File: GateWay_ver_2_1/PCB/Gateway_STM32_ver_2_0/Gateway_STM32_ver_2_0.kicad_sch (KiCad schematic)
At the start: 44 parts, among them J4 Conn_01x04, SW2 SW_Push, U7 STM32F407VETx, Y1 8mhz, Y2 Crystal_GND23

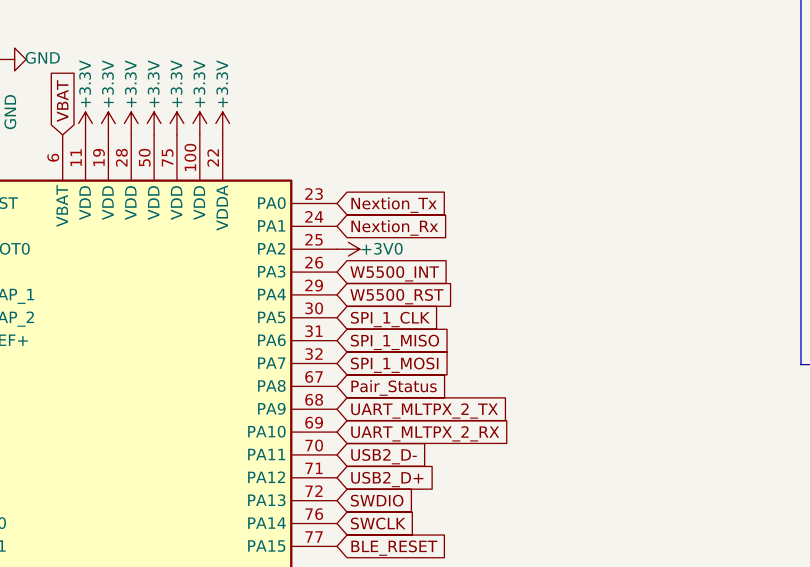
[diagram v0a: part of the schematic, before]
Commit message: 1
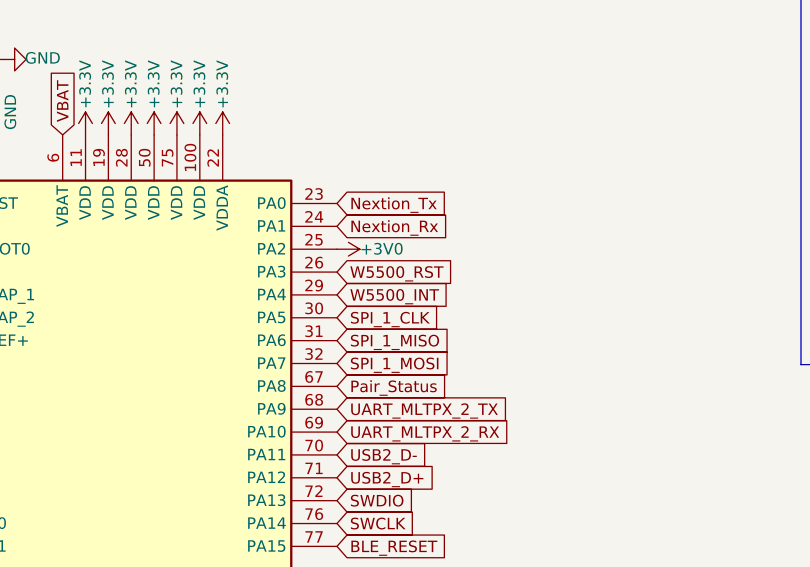
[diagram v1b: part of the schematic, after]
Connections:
- net W5500_INT: now also U7.29 (PA4); no longer U7.26 (PA3)
- net W5500_RST: now also U7.26 (PA3); no longer U7.29 (PA4)
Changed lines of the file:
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@@
     )
   )
-  (global_label "W5500_RST" (shape input) (at 114.046 61.468 0) (fields_autoplaced)
+  (global_label "W5500_RST" (shape input) (at 114.046 58.928 0) (fields_autoplaced)
     (effects (font (size 1.27 1.27)) (justify left))
-    (property "Intersheet References" "${INTERSHEET_REFS}" (id 0) (at 127.0745 61.5474 0)
+    (property "Intersheet References" "${INTERSHEET_REFS}" (id 0) (at 127.0745 59.0074 0)
       (effects (font (size 1.27 1.27)) (justify left) hide)
     )
@@
     )
   )
-  (global_label "W5500_INT" (shape input) (at 114.046 58.928 0) (fields_autoplaced)
+  (global_label "W5500_INT" (shape input) (at 114.046 61.468 0) (fields_autoplaced)
     (effects (font (size 1.27 1.27)) (justify left))
-    (property "Intersheet References" "${INTERSHEET_REFS}" (id 0) (at 126.5302 59.0074 0)
+    (property "Intersheet References" "${INTERSHEET_REFS}" (id 0) (at 126.5302 61.5474 0)
       (effects (font (size 1.27 1.27)) (justify left) hide)
     )
@@
       (reference "#PWR0291") (unit 1) (value "+3V0") (footprint "")
     )
+    (path "/8600ef7b-7ca3-4a98-82a9-dc0d4d9efebb/718c0a71-8caf-4775-a9fd-8fc71bd22381"
+      (reference "#PWR0292") (unit 1) (value "GND") (footprint "")
+    )
     (path "/17dbbc3f-e526-4f0c-aeef-1a51fbd344a5/44e527b0-0c19-4642-86b3-bad529530e43"
       (reference "#PWR0319") (unit 1) (value "+5V") (footprint "")
@@
       (reference "C27") (unit 1) (value "100uF") (footprint "Capacitor_SMD:C_1210_3225Metric")
     )
+    (path "/8600ef7b-7ca3-4a98-82a9-dc0d4d9efebb/57ebf0ae-ce32-4e87-bcc0-a3c92ff85e2b"
+      (reference "C28") (unit 1) (value "0.1uF") (footprint "Capacitor_SMD:C_0603_1608Metric")
+    )
     (path "/ddd7290c-9338-4156-8fc4-c8c1045ba903/431b55cc-a9c8-4999-8c91-373433ab34f0"
       (reference "C29") (unit 1) (value "0.1uF") (footprint "Capacitor_SMD:C_0603_1608Metric")
@@
       (reference "R93") (unit 1) (value "10k") (footprint "Resistor_SMD:R_0603_1608Metric")
     )
+    (path "/a04ecede-d1be-4f19-bba9-9cd40a161111/3f9a155b-ff8a-4cf2-8a3d-a6361ab24ec5"
+      (reference "R94") (unit 1) (value "0R") (footprint "Resistor_SMD:R_0603_1608Metric")
+    )
+    (path "/a04ecede-d1be-4f19-bba9-9cd40a161111/d410bbe8-62ea-4bf7-8bbe-58ba1610af3b"
+      (reference "R95") (unit 1) (value "0R") (footprint "Resistor_SMD:R_0603_1608Metric")
+    )
     (path "/dd619e6a-a0e1-4beb-8356-bcf75161c392/577f4706-5d40-4538-9616-d5b6ad5ea9f6"

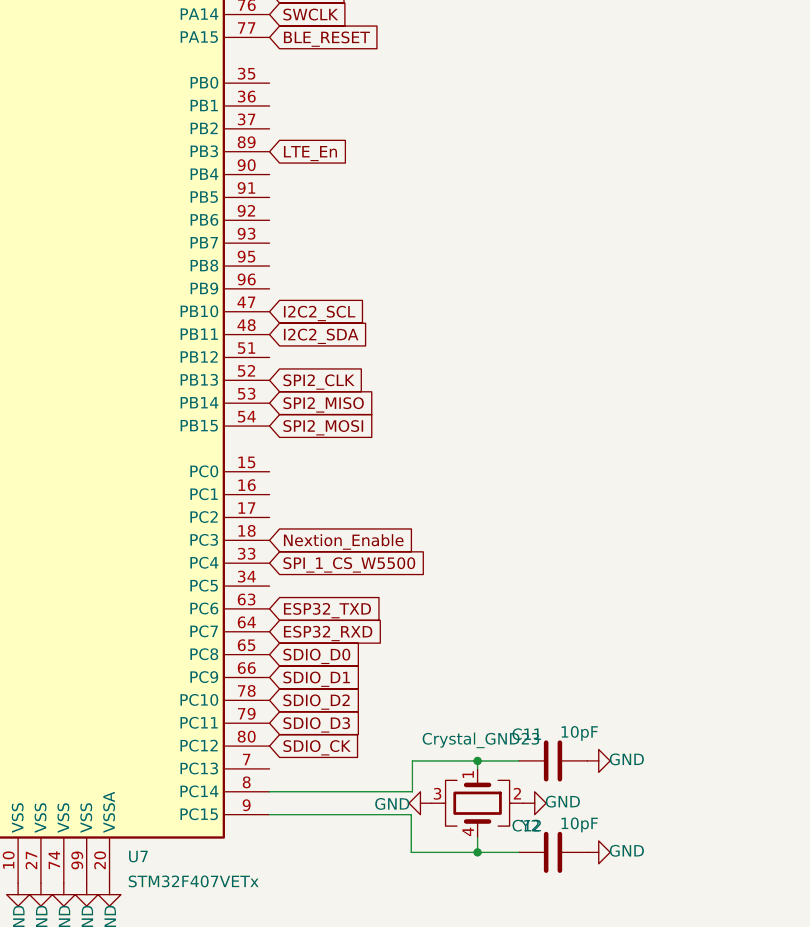
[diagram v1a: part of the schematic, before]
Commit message: 1
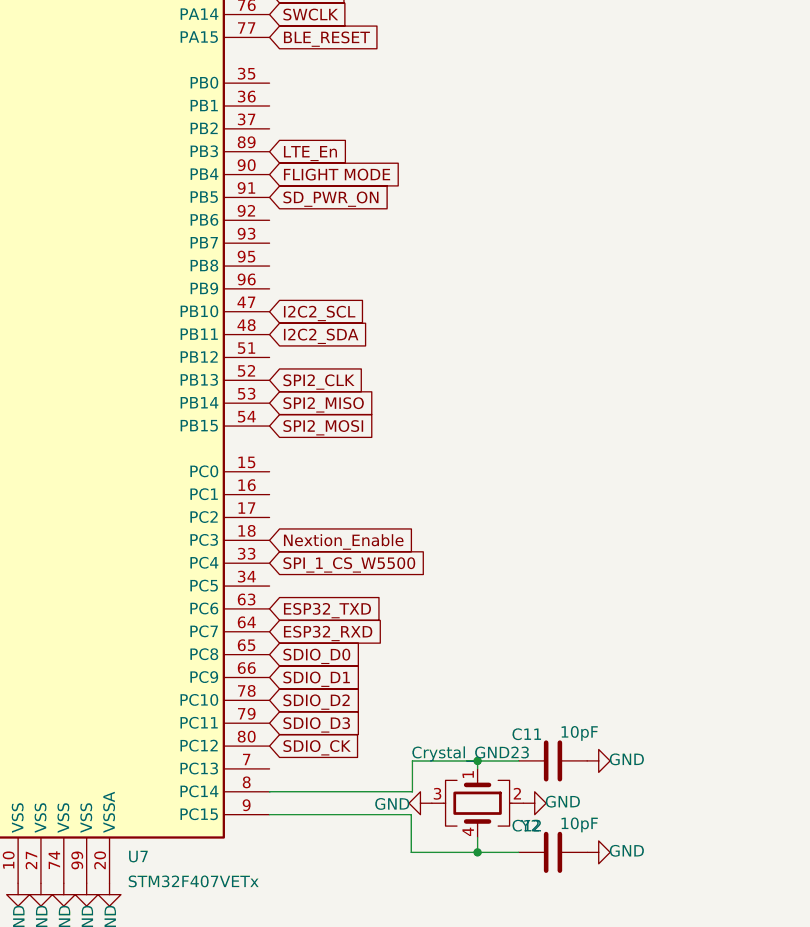
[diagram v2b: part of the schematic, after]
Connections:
- net FLIGHT MODE: now reaches U7.90 (PB4)
- net SD_PWR_ON: now reaches U7.91 (PB5)
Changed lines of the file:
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@@
     )
   )
+  (global_label "SD_PWR_ON" (shape input) (at 114.046 107.188 0) (fields_autoplaced)
+    (effects (font (size 1.27 1.27)) (justify left))
+    (property "Intersheet References" "${INTERSHEET_REFS}" (id 0) (at 127.4373 107.2674 0)
+      (effects (font (size 1.27 1.27)) (justify left) hide)
+    )
+  )
   (global_label "UART_MLTPX_1_RX" (shape input) (at 68.326 160.528 180) (fields_autoplaced)
     (effects (font (size 1.27 1.27)) (justify right))
@@
     )
   )
+  (global_label "FLIGHT MODE" (shape input) (at 114.046 104.648 0) (fields_autoplaced)
+    (effects (font (size 1.27 1.27)) (justify left))
+    (property "Intersheet References" "${INTERSHEET_REFS}" (id 0) (at 128.8283 104.7274 0)
+      (effects (font (size 1.27 1.27)) (justify left) hide)
+    )
+  )
   (global_label "UART_MLTPX_1_INH" (shape input) (at 68.326 170.688 180) (fields_autoplaced)
     (effects (font (size 1.27 1.27)) (justify right))
@@
       (effects (font (size 1.27 1.27)) (justify right))
     )
-    (property "Value" "Crystal_GND23" (id 1) (at 144.145 167.386 90)
+    (property "Value" "Crystal_GND23" (id 1) (at 143.002 168.91 90)
       (effects (font (size 1.27 1.27)) (justify right))
     )
@@
       (reference "#PWR0292") (unit 1) (value "GND") (footprint "")
     )
+    (path "/019ca31f-c666-4ad4-9da0-821bbd7be497/21b013d4-9869-46f8-91b4-c73f5a5d7438"
+      (reference "#PWR0293") (unit 1) (value "+1V8") (footprint "")
+    )
+    (path "/019ca31f-c666-4ad4-9da0-821bbd7be497/6b042a9e-5248-4333-84be-93a2e55bc491"
+      (reference "#PWR0294") (unit 1) (value "GND") (footprint "")
+    )
+    (path "/019ca31f-c666-4ad4-9da0-821bbd7be497/7441dc99-943a-4dad-884f-f78f21b79690"
+      (reference "#PWR0295") (unit 1) (value "GND") (footprint "")
+    )
+    (path "/019ca31f-c666-4ad4-9da0-821bbd7be497/be01e0c6-bdd6-4899-b88d-2ea45967df00"
+      (reference "#PWR0296") (unit 1) (value "GND") (footprint "")
+    )
+    (path "/1a27b42a-e314-45f7-981c-a9706a7662df/be407814-4163-4ebe-96a5-d393ad8660a1"
+      (reference "#PWR0297") (unit 1) (value "GND") (footprint "")
+    )
+    (path "/1a27b42a-e314-45f7-981c-a9706a7662df/d626ac88-2294-44a1-8045-a2014df7caaf"
+      (reference "#PWR0298") (unit 1) (value "GND") (footprint "")
+    )
+    (path "/1a27b42a-e314-45f7-981c-a9706a7662df/93b76a91-34ca-4e29-a20e-64701399a0a1"
+      (reference "#PWR0299") (unit 1) (value "GND") (footprint "")
+    )
+    (path "/1a27b42a-e314-45f7-981c-a9706a7662df/cb680b94-cb8a-403b-805b-635fdce1f75d"
+      (reference "#PWR0300") (unit 1) (value "+3.3V") (footprint "")
+    )
+    (path "/1a27b42a-e314-45f7-981c-a9706a7662df/81978b0a-e519-4d34-8933-65c54a8c622b"
+      (reference "#PWR0301") (unit 1) (value "+3.3V") (footprint "")
+    )
+    (path "/1a27b42a-e314-45f7-981c-a9706a7662df/54a7d9be-37e6-4e75-94ec-410902771d99"
+      (reference "#PWR0302") (unit 1) (value "+3.3V") (footprint "")
+    )
+    (path "/1a27b42a-e314-45f7-981c-a9706a7662df/ef7d2e66-f536-44d3-ab30-cf3ec18e9b70"
+      (reference "#PWR0303") (unit 1) (value "+3.3V") (footprint "")
+    )
+    (path "/1a27b42a-e314-45f7-981c-a9706a7662df/7e082b25-e0a3-4d23-815e-ffc0ae474c17"
+      (reference "#PWR0304") (unit 1) (value "+3.3V") (footprint "")
+    )
+    (path "/1a27b42a-e314-45f7-981c-a9706a7662df/dfdad1dd-3852-4e83-b7c5-23a3240fe4ae"
+      (reference "#PWR0305") (unit 1) (value "+3.3V") (footprint "")
+    )
+    (path "/1a27b42a-e314-45f7-981c-a9706a7662df/53559218-f782-43f3-8c33-3b9658ffab5a"
+      (reference "#PWR0306") (unit 1) (value "+3.3V") (footprint "")
+    )
+    (path "/1a27b42a-e314-45f7-981c-a9706a7662df/64422f56-284d-40c1-b987-146935e638d0"
+      (reference "#PWR0307") (unit 1) (value "GND") (footprint "")
+    )
+    (path "/1a27b42a-e314-45f7-981c-a9706a7662df/c98f6092-4097-47fd-be2a-78820fc284e9"
+      (reference "#PWR0308") (unit 1) (value "+3.3V") (footprint "")
+    )
+    (path "/1a27b42a-e314-45f7-981c-a9706a7662df/84b11d61-120c-4aff-8d74-1d997a30195e"
+      (reference "#PWR0309") (unit 1) (value "GND") (footprint "")
+    )
+    (path "/e0228e45-5e0c-439e-8ea8-5697529604dd/2969cfc9-b528-4fbf-858b-51587d5913c5"
+      (reference "#PWR0310") (unit 1) (value "+3.3V") (footprint "")
+    )
+    (path "/e0228e45-5e0c-439e-8ea8-5697529604dd/2c8b1a7a-111a-41a7-b837-a1f4012c4e65"
+      (reference "#PWR0311") (unit 1) (value "+3.3V") (footprint "")
+    )
     (path "/17dbbc3f-e526-4f0c-aeef-1a51fbd344a5/44e527b0-0c19-4642-86b3-bad529530e43"
       (reference "#PWR0319") (unit 1) (value "+5V") (footprint "")
@@
       (reference "#PWR0339") (unit 1) (value "GND") (footprint "")
     )
-    (path "/1a27b42a-e314-45f7-981c-a9706a7662df/9ded5ff0-8d1a-49a0-aa65-89c230ed4d38"
-      (reference "#PWR0340") (unit 1) (value "+3.3V") (footprint "")
-    )
     (path "/1a27b42a-e314-45f7-981c-a9706a7662df/8f08bab3-f095-4448-ac94-d3d0aeb31d03"
       (reference "#PWR0341") (unit 1) (value "GND") (footprint "")
@@
       (reference "C110") (unit 1) (value "0.1uF") (footprint "Capacitor_SMD:C_0603_1608Metric")
     )
+    (path "/019ca31f-c666-4ad4-9da0-821bbd7be497/4431fc22-802c-454c-be8c-6a5409044ac5"
+      (reference "C111") (unit 1) (value "22pF") (footprint "Capacitor_SMD:C_0603_1608Metric")
+    )
+    (path "/019ca31f-c666-4ad4-9da0-821bbd7be497/7229f3de-f2e5-463b-b798-c5991fbed455"
+      (reference "C112") (unit 1) (value "0.1uF") (footprint "Capacitor_SMD:C_0603_1608Metric")
+    )
+    (path "/019ca31f-c666-4ad4-9da0-821bbd7be497/035ea0ca-09f0-47d6-8803-a4d3d340ae9a"
+      (reference "C113") (unit 1) (value "33pF") (footprint "Capacitor_SMD:C_0603_1608Metric")
+    )
+    (path "/1a27b42a-e314-45f7-981c-a9706a7662df/33872170-1318-49d3-a9cf-aabd45781f4f"
+      (reference "C114") (unit 1) (value "10uF") (footprint "Capacitor_SMD:C_0805_2012Metric")
+    )
     (path "/c160f45b-9b3f-4634-96f2-f5447d1e210d"
       (reference "D1") (unit 1) (value "1N5819") (footprint "Footprint:SOD-323")
@@
       (reference "Q8") (unit 1) (value "MMBT3906") (footprint "Package_TO_SOT_SMD:SOT-23")
     )
+    (path "/019ca31f-c666-4ad4-9da0-821bbd7be497/01b6de27-d803-489f-8d79-a2a2cb7090fe"
+      (reference "Q9") (unit 1) (value "AO3400") (footprint "Package_TO_SOT_SMD:SOT-23")
+    )
     (path "/ddd7290c-9338-4156-8fc4-c8c1045ba903/b3051a5e-cd79-401b-8db6-8cc2119ff835"
       (reference "R1") (unit 1) (value "12k") (footprint "Resistor_SMD:R_0603_1608Metric")
@@
       (reference "R95") (unit 1) (value "0R") (footprint "Resistor_SMD:R_0603_1608Metric")
     )
+    (path "/019ca31f-c666-4ad4-9da0-821bbd7be497/8b7d305c-caee-4338-94fc-4790d784af7f"
+      (reference "R96") (unit 1) (value "4.7k") (footprint "Resistor_SMD:R_0603_1608Metric")
+    )
+    (path "/019ca31f-c666-4ad4-9da0-821bbd7be497/18a82b42-2202-42c2-bf5c-5f6ee35bca85"
+      (reference "R97") (unit 1) (value "4.7k") (footprint "Resistor_SMD:R_0603_1608Metric")
+    )
+    (path "/019ca31f-c666-4ad4-9da0-821bbd7be497/10df4dce-a0b7-467b-a44d-149fa24d1a83"
+      (reference "R98") (unit 1) (value "47k") (footprint "Resistor_SMD:R_0603_1608Metric")
+    )
+    (path "/1a27b42a-e314-45f7-981c-a9706a7662df/84c55e87-ec53-4ed2-bf44-c407a0315a34"
+      (reference "R99") (unit 1) (value "10k") (footprint "Resistor_SMD:R_0603_1608Metric")
+    )
+    (path "/1a27b42a-e314-45f7-981c-a9706a7662df/850acc6f-fe0b-468c-85e1-9fc39955f1b1"
+      (reference "R100") (unit 1) (value "10k") (footprint "Resistor_SMD:R_0603_1608Metric")
+    )
+    (path "/1a27b42a-e314-45f7-981c-a9706a7662df/7d8f48d2-427b-401f-85c8-33bdeab8224d"
+      (reference "R101") (unit 1) (value "10k") (footprint "Resistor_SMD:R_0603_1608Metric")
+    )
+    (path "/1a27b42a-e314-45f7-981c-a9706a7662df/a2c2f513-fcf4-42c3-a1d6-81d1a365be99"
+      (reference "R102") (unit 1) (value "10k") (footprint "Resistor_SMD:R_0603_1608Metric")
+    )
+    (path "/1a27b42a-e314-45f7-981c-a9706a7662df/3cfb438a-7745-48ec-bb55-3c4dcc7aa34d"
+      (reference "R103") (unit 1) (value "10k") (footprint "Resistor_SMD:R_0603_1608Metric")
+    )
+    (path "/1a27b42a-e314-45f7-981c-a9706a7662df/e2ae9604-d9ea-4f7f-95c7-d2f91f7a1207"
+      (reference "R104") (unit 1) (value "10k") (footprint "Resistor_SMD:R_0603_1608Metric")
+    )
+    (path "/1a27b42a-e314-45f7-981c-a9706a7662df/0e44764b-f330-45d6-8e49-eb46d4e6dcfb"
+      (reference "R105") (unit 1) (value "10k") (footprint "Resistor_SMD:R_0603_1608Metric")
+    )
+    (path "/e0228e45-5e0c-439e-8ea8-5697529604dd/da97e812-19af-46bb-b1f4-df65d07d9b19"
+      (reference "R106") (unit 1) (value "10k") (footprint "Resistor_SMD:R_0603_1608Metric")
+    )
+    (path "/e0228e45-5e0c-439e-8ea8-5697529604dd/3d1b0045-da5c-4ca7-8b48-14fb5f9aee36"
+      (reference "R107") (unit 1) (value "10k") (footprint "Resistor_SMD:R_0603_1608Metric")
+    )
     (path "/dd619e6a-a0e1-4beb-8356-bcf75161c392/577f4706-5d40-4538-9616-d5b6ad5ea9f6"
       (reference "SW1") (unit 1) (value "SW_Push") (footprint "Button_Switch_SMD:SW_SPST_CK_RS282G05A3")
@@
       (reference "U21") (unit 1) (value "TPS2041C") (footprint "Package_TO_SOT_SMD:SOT-23-5")
     )
+    (path "/1a27b42a-e314-45f7-981c-a9706a7662df/081d1ce9-d69c-4cef-b14c-fb7e8e25b79d"
+      (reference "U22") (unit 1) (value "TPD2EUSB30") (footprint "Package_TO_SOT_SMD:Texas_DRT-3")
+    )
+    (path "/1a27b42a-e314-45f7-981c-a9706a7662df/c0f456cc-124b-4394-9b21-99df35bf4230"
+      (reference "U23") (unit 1) (value "TPD2EUSB30") (footprint "Package_TO_SOT_SMD:Texas_DRT-3")
+    )
+    (path "/1a27b42a-e314-45f7-981c-a9706a7662df/cf3b9950-37ce-4a5a-8a21-fa72b624af22"
+      (reference "U24") (unit 1) (value "TPD2EUSB30") (footprint "Package_TO_SOT_SMD:Texas_DRT-3")
+    )
+    (path "/1a27b42a-e314-45f7-981c-a9706a7662df/f30a38a6-df38-4442-83eb-9c7b9f1a32a6"
+      (reference "U25") (unit 1) (value "RT9742AGJ5F") (footprint "Package_TO_SOT_SMD:TSOT-23-5")
+    )
     (path "/8832c854-dd5b-4a42-8207-a65f82d7dd7a"
